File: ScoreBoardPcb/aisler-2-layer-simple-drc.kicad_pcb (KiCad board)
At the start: 2 copper layers, 58.8 x 67.1 mm, 16 parts, among them J1 Conn_02x20_Odd_Even, U1 CD74HCT4066M96, U2 CD74HCT4066M96, U3 CD74HCT4066M96, U5 ADM3101EARQZ-REEL

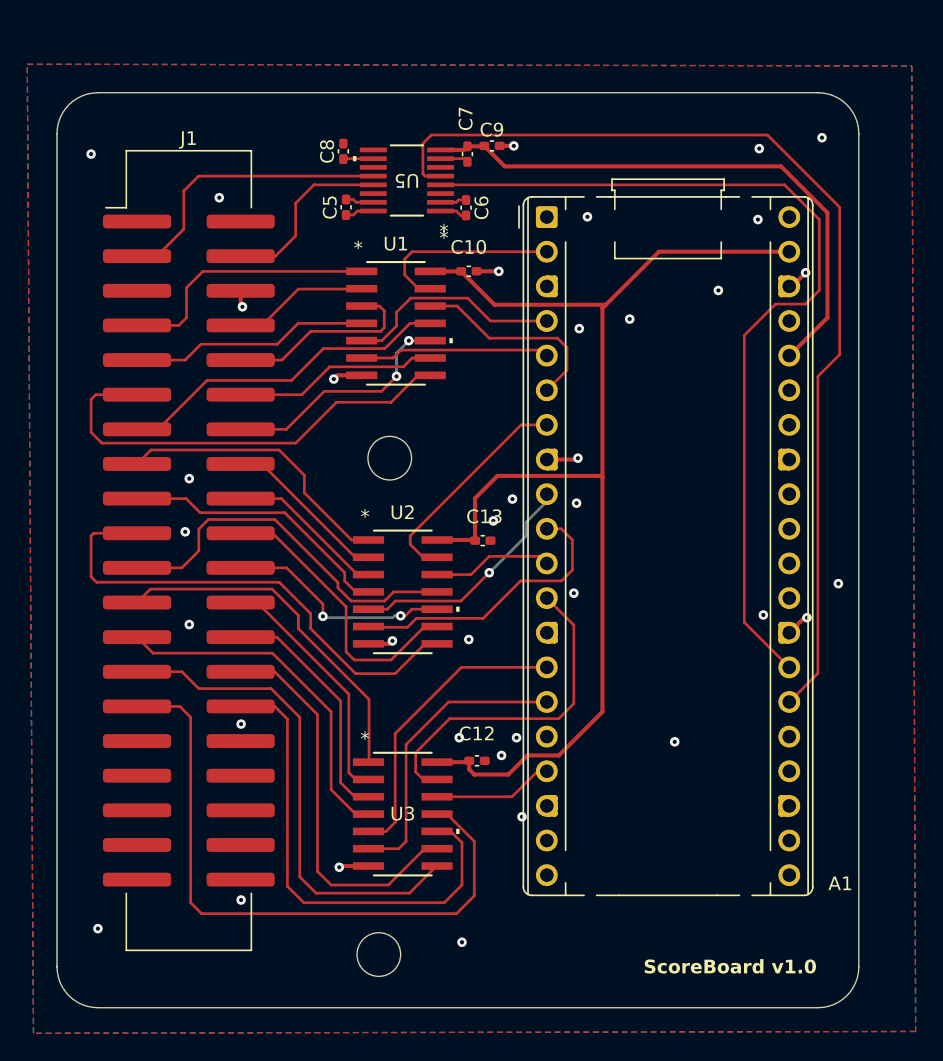
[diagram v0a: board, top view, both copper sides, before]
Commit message: Rev 1.0 submitted for manf
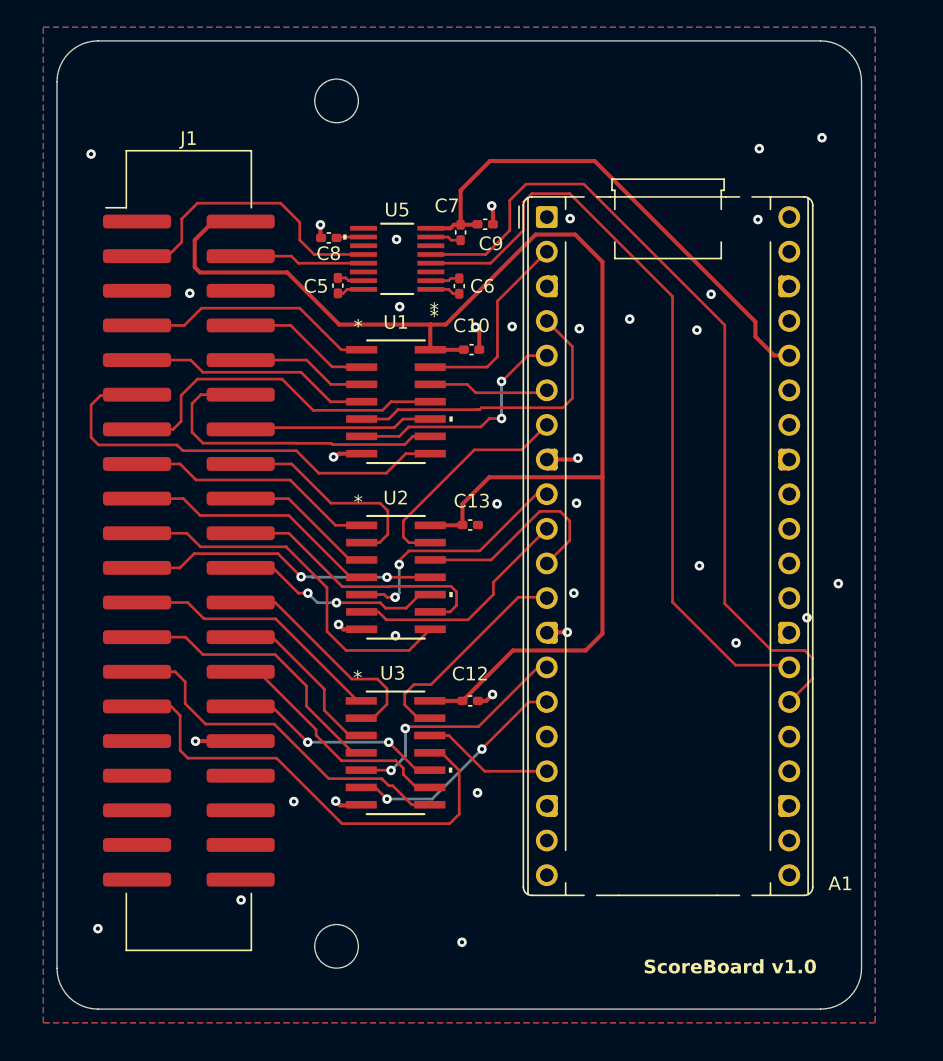
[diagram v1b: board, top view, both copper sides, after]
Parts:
- A1: footprint Module:RaspberryPi_Pico_Common_THT -> ScoreBoardPcb:RaspberryPi_Pico_Common_THT
- moved H1 26.5 mm to (120.5, 54.4)
- moved C8 6.44 mm to (119.9, 64.4), turned to 180 degrees
- moved U5 5.79 mm to (124.9, 66.0)
- moved C5 5.78 mm to (120.6, 67.9)
- moved C6 5.77 mm to (129.5, 68.0)
- moved C7 5.77 mm to (129.6, 64.0)
- moved C9 5.77 mm to (131.4, 63.4)
- moved C10 5.75 mm to (130.4, 72.6)
- moved U1 5.75 mm to (124.9, 76.5)
- moved U3 4.52 mm to (124.8, 102.2)
- moved C12 4.42 mm to (130.3, 98.4)
- moved H2 3.16 mm to (120.5, 116.4)
- moved C13 1.47 mm to (130.3, 85.5)
- moved U2 1.18 mm to (124.9, 89.3)
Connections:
- A1 pad 39: +5V -> unconnected-(A1-VSYS-Pad39)
- J1 pad 2: GND -> +5V
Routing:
- net /AUX_2: track 34.2 -> 12.6 mm, vias 0 -> 2
- net /TX_TTL: track 74.4 -> 61.7 mm
- net /AUX_1: track 46.4 -> 34.0 mm
- net /CLEAR_2: track 27.8 -> 15.6 mm
- net +5V: track 89.6 -> 100.4 mm
- net /CLEAR_1: track 36.4 -> 26.4 mm
- net /RX_TTL: track 66.6 -> 56.9 mm
- net /HOME_DEC_2: track 15.0 -> 24.0 mm
- net /SEC_INC: track 23.8 -> 15.5 mm
- net /MIN_INC_1: track 35.4 -> 27.6 mm
- net /MIN_DEC: track 8.86 -> 15.8 mm
- net /SEC_DEC_2: track 16.4 -> 9.55 mm
- net /SEC_INC_1: track 26.0 -> 19.2 mm
- net /AWAY_DEC_2: track 9.68 -> 16.1 mm
- net /AWAY_INC: track 15.0 -> 8.62 mm
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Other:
- board size 58.8 x 67.1 mm -> 59 x 71 mm
